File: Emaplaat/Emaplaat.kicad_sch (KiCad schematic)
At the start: 18 parts, among them IC2 ESP32-S3-WROOM-2-N32R16V, J2 Screw_Terminal_01x02, J3 Conn_01x09_Pin, J4 Conn_01x09_Pin, J7 Screw_Terminal_01x02, Q1 2N7002K

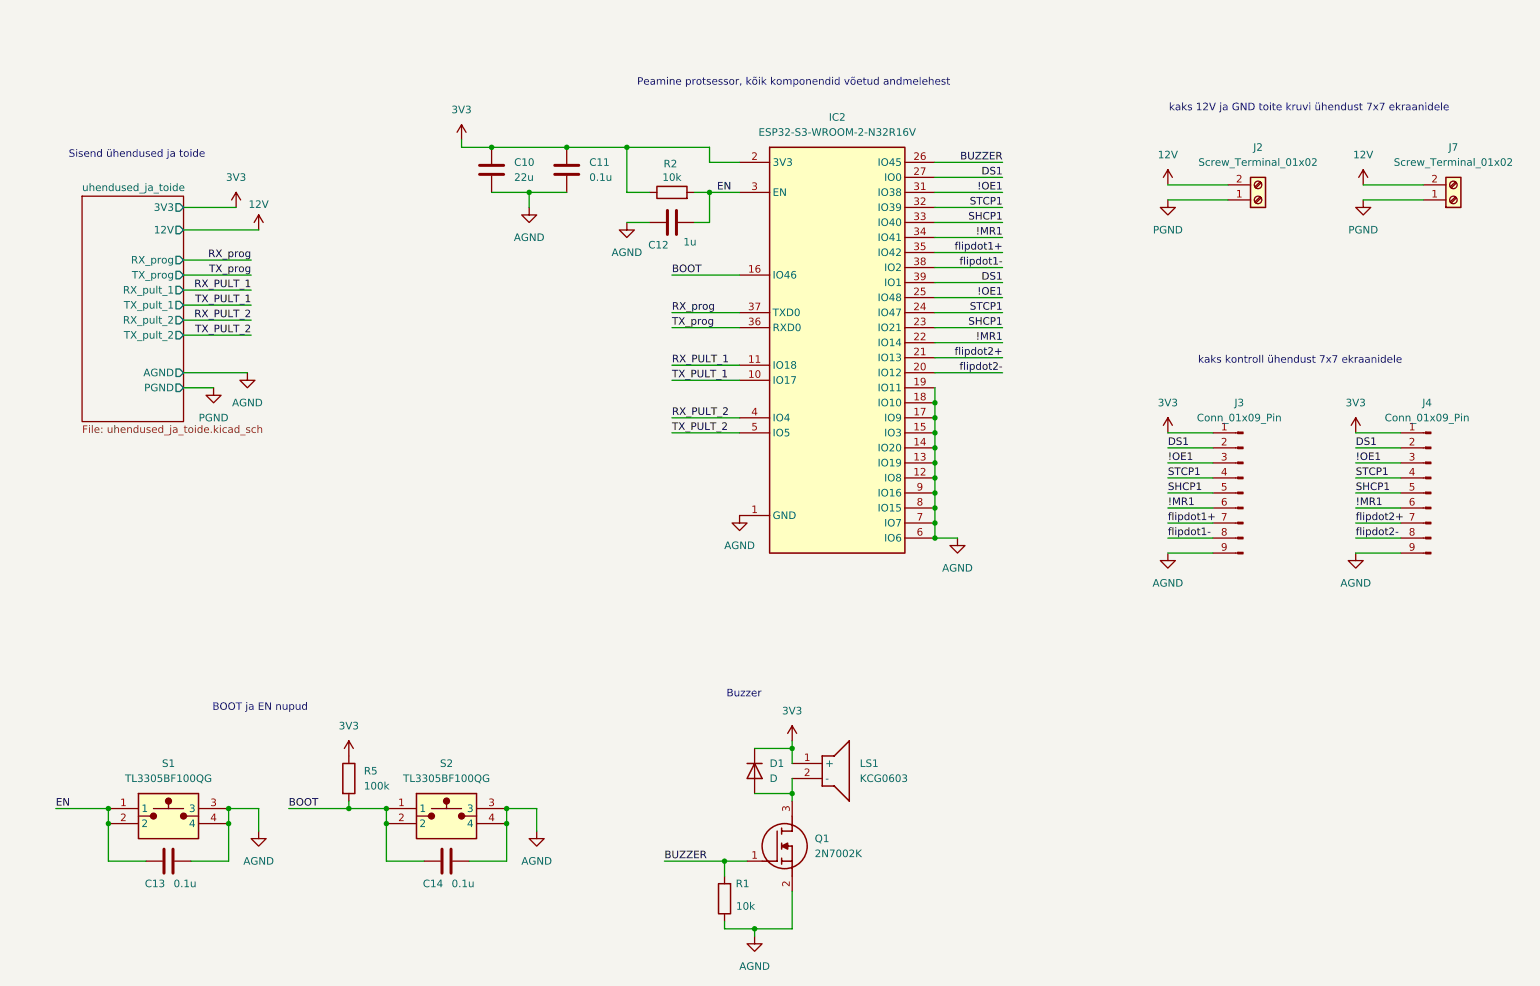
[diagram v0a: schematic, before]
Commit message: qwerghhgfdsdfghqwerghhgfdsdfghjj
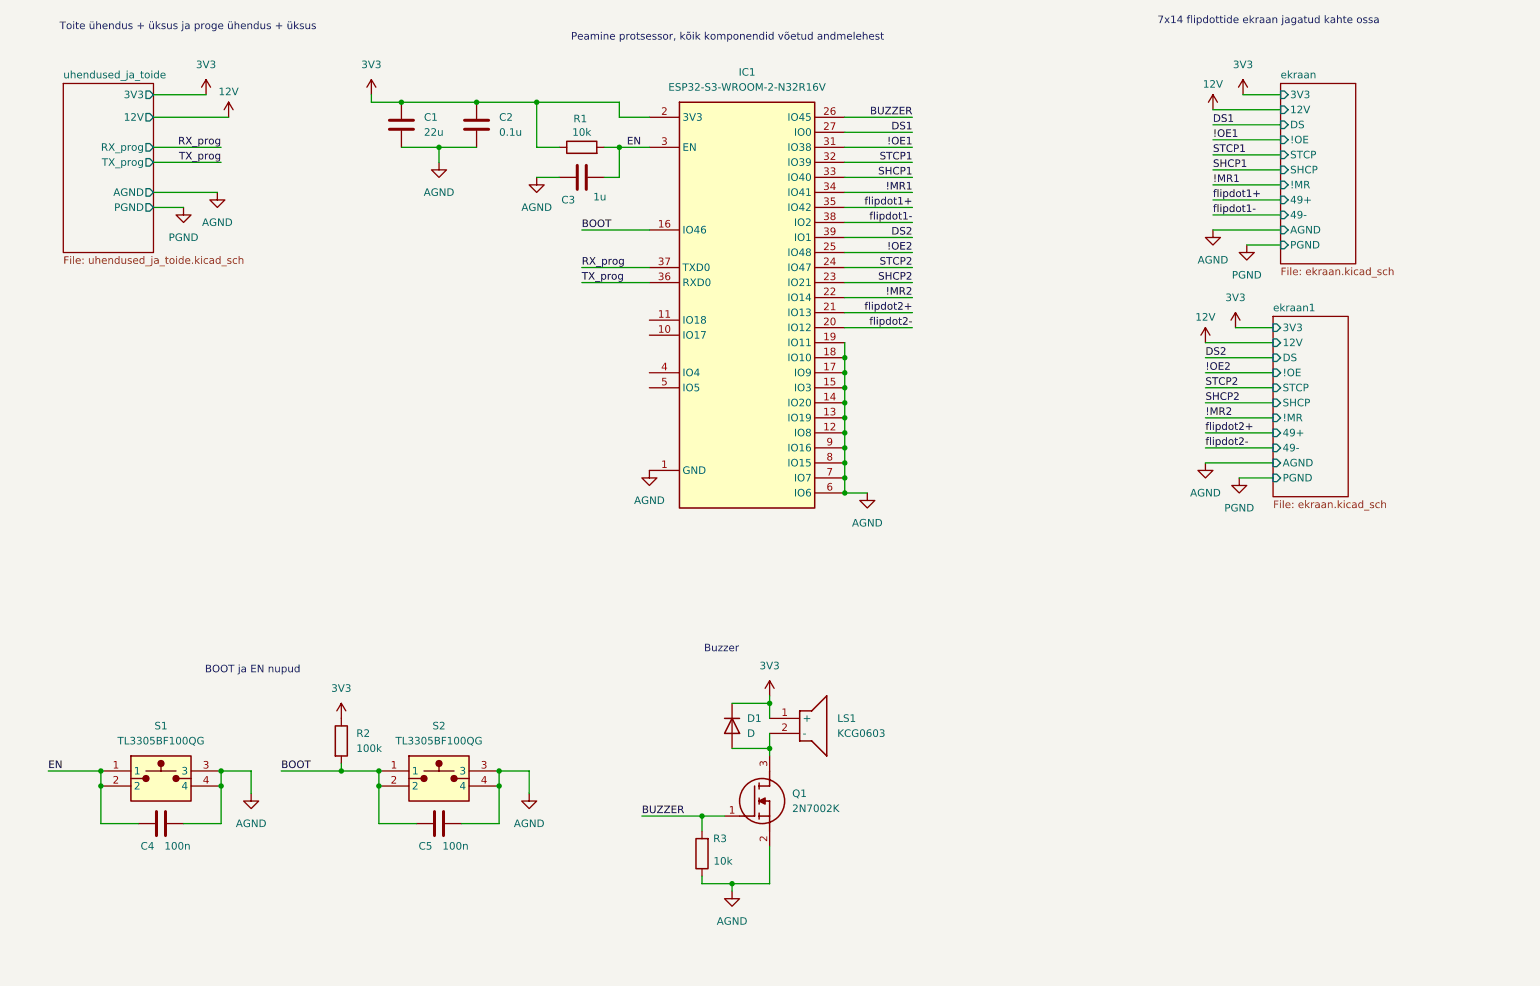
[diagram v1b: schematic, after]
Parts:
- removed J2, J7: Screw_Terminal_01x02, symbol Connector:Screw_Terminal_01x02
- removed J3, J4: Conn_01x09_Pin, symbol Connector:Conn_01x09_Pin
- C4: renamed from C13; value 0.1u -> 100n
- C5: renamed from C14; value 0.1u -> 100n
- renumbered C10 to C1, C11 to C2, C12 to C3, IC2 to IC1, R2 to R1, R5 to R2, R1 to R3
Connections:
- net !MR1: no longer IC1.22 (IO14)
- net !OE1: no longer IC1.25 (IO48)
- net DS1: no longer IC1.39 (IO1)
- net SHCP1: no longer IC1.23 (IO21)
- net STCP1: no longer IC1.24 (IO47)
- net RX_PULT_1: no longer names the net of IC1.11 (IO18)
- net RX_PULT_2: no longer names the net of IC1.4 (IO4)
- net TX_PULT_1: no longer names the net of IC1.10 (IO17)
- net TX_PULT_2: no longer names the net of IC1.5 (IO5)
- new net !MR2: IC1.22 (IO14)
- new net !OE2: IC1.25 (IO48)
- new net DS2: IC1.39 (IO1)
- new net SHCP2: IC1.23 (IO21)
- new net STCP2: IC1.24 (IO47)
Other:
- added sheet ekraan (ekraan.kicad_sch)
- added sheet ekraan1 (ekraan.kicad_sch)
- sheet uhendused_ja_toide ports: added none; removed RX_pult_1, RX_pult_2, TX_pult_1, TX_pult_2
- note added: "7x14 flipdottide ekraan jagatud kahte ossa"
- note added: "Toite ühendus + üksus ja proge ühendus + üksus"
- note removed: "Sisend ühendused ja toide"
- note removed: "kaks 12V ja GND toite kruvi ühendust 7x7 ekraanidele"
- note removed: "kaks kontroll ühendust 7x7 ekraanidele"
- moved on the sheet: C1, C2, C3, C4, C5, D1, IC1, LS1, Q1, R1, R2, R3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

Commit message: fliptendo gameboy type shi
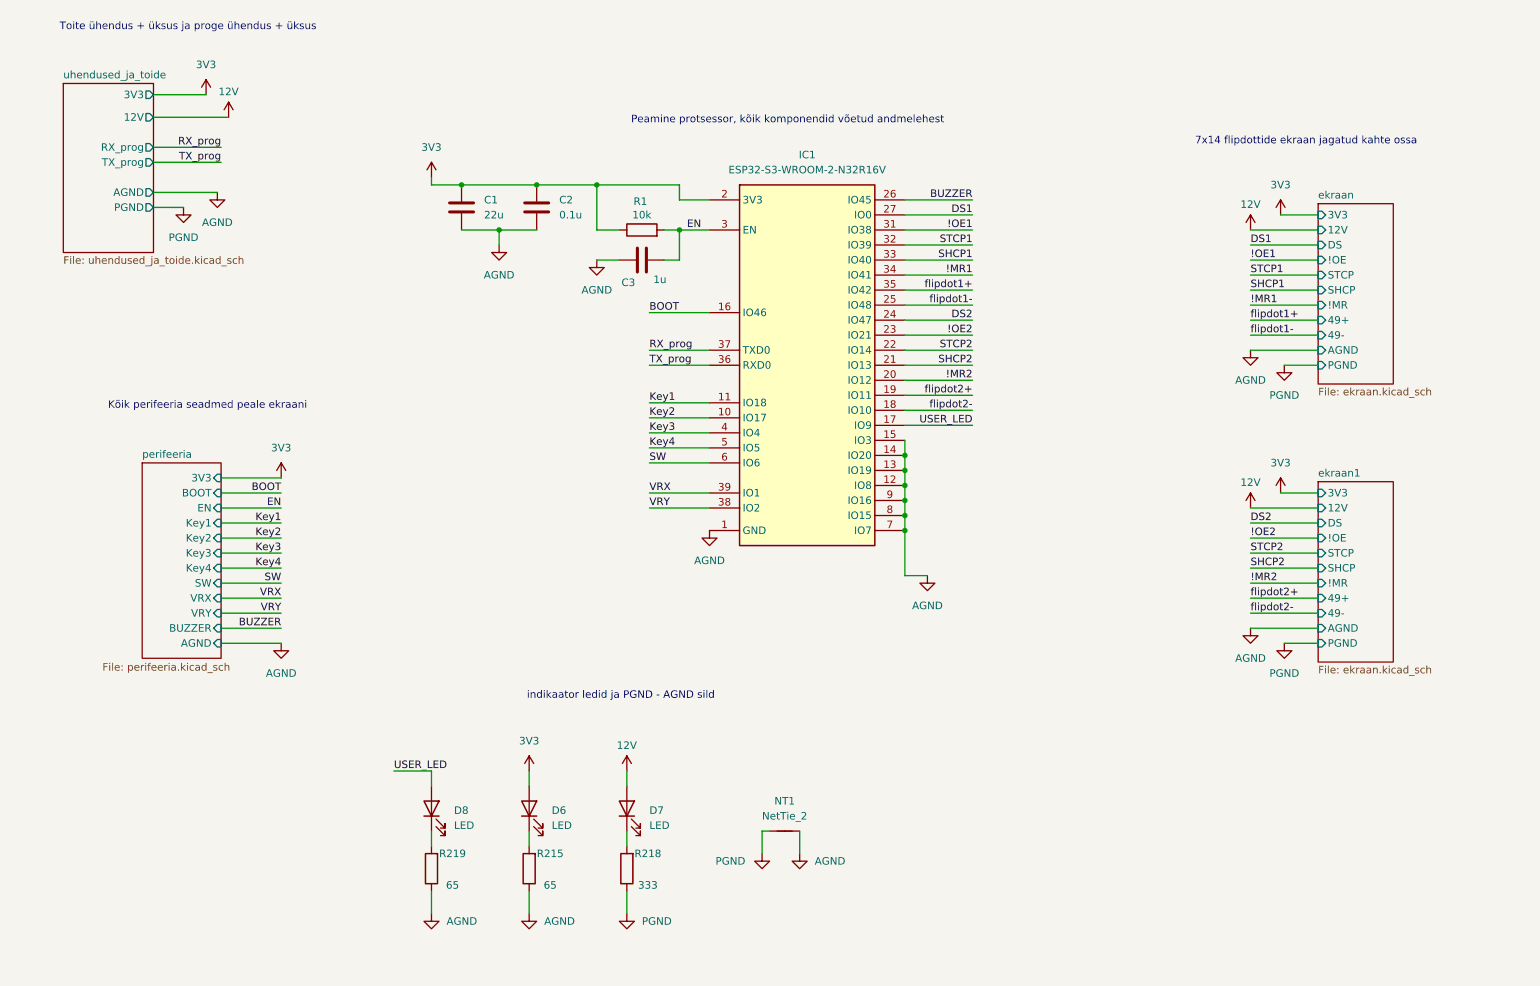
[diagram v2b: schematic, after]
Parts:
- removed C4, C5: 100n, symbol Device:C
- removed D1: D, symbol Device:D
- removed LS1: KCG0603, KCG0603, symbol KCG0603:KCG0603
- removed Q1: 2N7002K, SOT95P240X120-3N, symbol 2N7002K:2N7002K
- removed R2: 100k, symbol Device:R
- removed R3: 10k, symbol Device:R
- removed S1, S2: TL3305BF100QG, TL3305BF160QG, symbol TL3305BF100QG:TL3305BF100QG
- added D6, D7, D8: LED, LED_SMD:LED_0603_1608Metric, symbol Device:LED
- added NT1: NetTie_2, NetTie:NetTie-2_SMD_Pad0.5mm, symbol Device:NetTie_2
- added R215, R219: 65, Resistor_SMD:R_0603_1608Metric, symbol Device:R
- added R218: 333, Resistor_SMD:R_0603_1608Metric, symbol Device:R
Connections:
- net !MR2: now also IC1.20 (IO12); no longer IC1.22 (IO14)
- net !OE2: now also IC1.23 (IO21); no longer IC1.25 (IO48)
- net 12V: now also D7.2 (A)
- net 3V3: now also D6.2 (A)
- net AGND: now also NT1.2, R215.1, R219.1; no longer IC1.17 (IO9), IC1.18 (IO10), IC1.19 (IO11), IC1.6 (IO6)
- net DS2: now also IC1.24 (IO47); no longer IC1.39 (IO1)
- net PGND: now also NT1.1, R218.1
- net SHCP2: now also IC1.21 (IO13); no longer IC1.23 (IO21)
- net STCP2: now also IC1.22 (IO14); no longer IC1.24 (IO47)
- net flipdot1-: now also IC1.25 (IO48); no longer IC1.38 (IO2)
- net flipdot2+: now also IC1.19 (IO11); no longer IC1.21 (IO13)
- net flipdot2-: now also IC1.18 (IO10); no longer IC1.20 (IO12)
- net Key2: now reaches IC1.10 (IO17)
- net Key1: now reaches IC1.11 (IO18)
- net Key3: now reaches IC1.4 (IO4)
- net Key4: now reaches IC1.5 (IO5)
- new net: D8.1 (K), R219.2
- new net: D6.1 (K), R215.2
- new net: D7.1 (K), R218.2
- new net SW: IC1.6 (IO6)
- new net USER_LED: D8.2 (A), IC1.17 (IO9)
- new net VRX: IC1.39 (IO1)
- new net VRY: IC1.38 (IO2)
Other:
- added sheet perifeeria (perifeeria.kicad_sch)
- note added: "Kõik perifeeria seadmed peale ekraani"
- note added: "indikaator ledid ja PGND - AGND sild"
- note removed: "BOOT ja EN nupud"
- note removed: "Buzzer"
- moved on the sheet: C1, C2, C3, IC1, R1
